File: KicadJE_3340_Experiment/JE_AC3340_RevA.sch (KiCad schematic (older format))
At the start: 89 parts

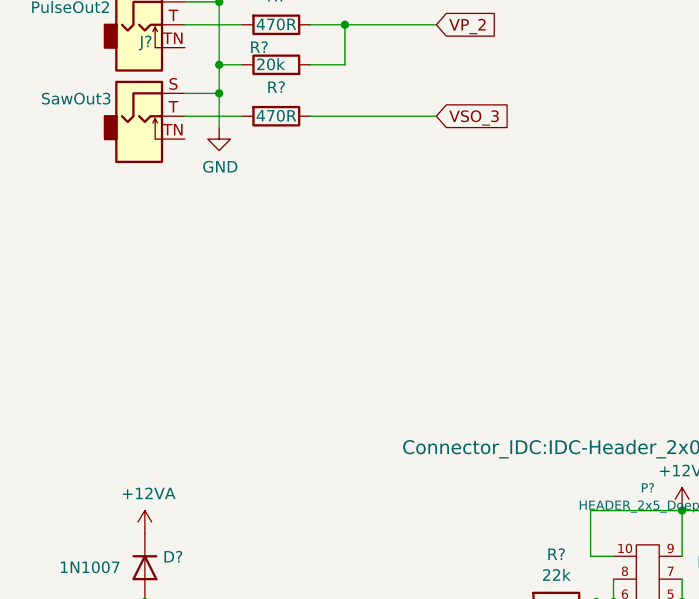
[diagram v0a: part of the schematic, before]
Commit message: Octave switch JE
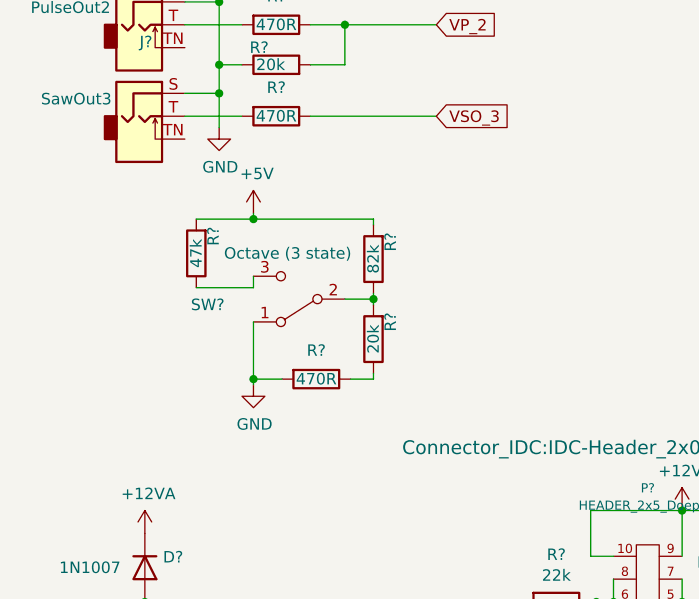
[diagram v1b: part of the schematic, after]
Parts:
- added R?: 82k, Resistor_SMD:R_0805_2012Metric_Pad1.15x1.40mm_HandSolder, symbol Device:R
- added R?: 20k, Resistor_SMD:R_0805_2012Metric_Pad1.15x1.40mm_HandSolder, symbol Device:R
- added R?: 47k, Resistor_SMD:R_0805_2012Metric_Pad1.15x1.40mm_HandSolder, symbol Device:R
- added R?: 470R, Resistor_SMD:R_0805_2012Metric_Pad1.15x1.40mm_HandSolder, symbol Device:R
- added SW?: Octave (3 state), AJ-Dropbox-Kicad:SP1MS1, symbol Switch:SW_SPDT
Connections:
- net +5V: now also R?.2, R?.2
- net GND: now also R?.2, SW?.1 (A)
- new net: R?.1, R?.2, SW?.2 (B)
- new net: R?.1, SW?.3 (C)
- new net: R?.1, R?.1
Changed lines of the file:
@@
 AR Path="/5E4B0DD9/5F66CD2B" Ref="U?"  Part="1"
 AR Path="/5E62ACA1/5F66CD2B" Ref="U?"  Part="1"
+AR Path="/5F49A670/5F66CD2B" Ref="U?"  Part="1"
 F 0 "U?" H 10300 4631 50  0000 C CNN
 F 1 "AS3340" H 10300 4540 50  0000 C CNN
@@
 AR Path="/5E4B0DD9/5F66CD3F" Ref="C?"  Part="1"
 AR Path="/5E62ACA1/5F66CD3F" Ref="C?"  Part="1"
+AR Path="/5F49A670/5F66CD3F" Ref="C?"  Part="1"
 F 0 "C?" H 9200 4450 50  0000 L CNN
 F 1 "1n poly" H 9125 4200 50  0000 L CNN
@@
 AR Path="/5E4B0DD9/5F66CD4A" Ref="R?"  Part="1"
 AR Path="/5E62ACA1/5F66CD4A" Ref="R?"  Part="1"
+AR Path="/5F49A670/5F66CD4A" Ref="R?"  Part="1"
 F 0 "R?" V 9550 4450 50  0000 C CNN
 F 1 "1k82" V 9675 4450 50  0000 C CNN
@@
 AR Path="/5E4B0DD9/5F66CD58" Ref="#PWR?"  Part="1"
 AR Path="/5E62ACA1/5F66CD58" Ref="#PWR?"  Part="1"
+AR Path="/5F49A670/5F66CD58" Ref="#PWR?"  Part="1"
 F 0 "#PWR?" H 9425 4400 50  0001 C CNN
 F 1 "GND" H 9430 4477 50  0000 C CNN
@@
 AR Path="/5E4B0DD9/5F66CD63" Ref="R?"  Part="1"
 AR Path="/5E62ACA1/5F66CD63" Ref="R?"  Part="1"
+AR Path="/5F49A670/5F66CD63" Ref="R?"  Part="1"
 F 0 "R?" V 9375 3400 50  0000 C CNN
 F 1 "6k04" V 9425 3250 50  0000 C CNN
@@
 AR Path="/5E4B0DD9/5F66CD69" Ref="R?"  Part="1"
 AR Path="/5E62ACA1/5F66CD69" Ref="R?"  Part="1"
+AR Path="/5F49A670/5F66CD69" Ref="R?"  Part="1"
 F 0 "R?" V 9325 3275 50  0000 C CNN
 F 1 "26k7" V 9425 3150 50  0000 C CNN
@@
 AR Path="/5E4B0DD9/5F66CD6F" Ref="RV?"  Part="1"
 AR Path="/5E62ACA1/5F66CD6F" Ref="RV?"  Part="1"
+AR Path="/5F49A670/5F66CD6F" Ref="RV?"  Part="1"
 F 0 "RV?" V 9150 3050 50  0000 C CNN
 F 1 "5k" V 9025 3175 50  0000 C CNN
@@
 AR Path="/5E4B0DD9/5F66CD7D" Ref="#PWR?"  Part="1"
 AR Path="/5E62ACA1/5F66CD7D" Ref="#PWR?"  Part="1"
+AR Path="/5F49A670/5F66CD7D" Ref="#PWR?"  Part="1"
 F 0 "#PWR?" H 10400 4350 50  0001 C CNN
 F 1 "GND" H 10405 4427 50  0000 C CNN
@@
 AR Path="/5E4B0DD9/5F66CD91" Ref="R?"  Part="1"
 AR Path="/5E62ACA1/5F66CD91" Ref="R?"  Part="1"
+AR Path="/5F49A670/5F66CD91" Ref="R?"  Part="1"
 F 0 "R?" V 9375 3500 50  0000 C CNN
 F 1 "1M2" V 9425 3350 50  0000 C CNN
@@
 U 1 1 5F66CD99
 P 8675 3150
+AR Path="/5E62ACA1/5F66CD99" Ref="#PWR?"  Part="1"
+AR Path="/5F49A670/5F66CD99" Ref="#PWR?"  Part="1"
 F 0 "#PWR?" H 8675 3250 50  0001 C CNN
 F 1 "-5V" H 8690 3323 50  0000 C CNN
@@
 AR Path="/5E4B0DD9/5F66CD9F" Ref="#PWR?"  Part="1"
 AR Path="/5E62ACA1/5F66CD9F" Ref="#PWR?"  Part="1"
+AR Path="/5F49A670/5F66CD9F" Ref="#PWR?"  Part="1"
 F 0 "#PWR?" H 9125 3225 50  0001 C CNN
 F 1 "-12VA" H 9140 3548 50  0000 C CNN
@@
 AR Path="/5F18E4B5/5F66CDA9" Ref="C?"  Part="1"
 AR Path="/5E62ACA1/5F66CDA9" Ref="C?"  Part="1"
+AR Path="/5F49A670/5F66CDA9" Ref="C?"  Part="1"
 F 0 "C?" H 8925 4450 50  0000 L CNN
 F 1 "100n" H 8850 4275 50  0000 L CNN
@@
 U 1 1 5F66CDB6
 P 10300 4625
+AR Path="/5E62ACA1/5F66CDB6" Ref="#PWR?"  Part="1"
+AR Path="/5F49A670/5F66CDB6" Ref="#PWR?"  Part="1"
 F 0 "#PWR?" H 10300 4725 50  0001 C CNN
 F 1 "-5V" H 10315 4798 50  0000 C CNN
@@
 U 1 1 5F66CDBC
 P 8550 3950
+AR Path="/5E62ACA1/5F66CDBC" Ref="Q?"  Part="1"
+AR Path="/5F49A670/5F66CDBC" Ref="Q?"  Part="1"
 F 0 "Q?" H 8741 3904 50  0000 L CNN
 F 1 "MMBT3906" H 8741 3995 50  0000 L CNN
@@
 AR Path="/5E4B0DD9/5F66CDC3" Ref="C?"  Part="1"
 AR Path="/5E62ACA1/5F66CDC3" Ref="C?"  Part="1"
+AR Path="/5F49A670/5F66CDC3" Ref="C?"  Part="1"
 F 0 "C?" V 7550 4150 50  0000 L CNN
 F 1 "220p" V 7650 4150 50  0000 L CNN
@@
 AR Path="/5E4B0DD9/5F66CDC9" Ref="R?"  Part="1"
 AR Path="/5E62ACA1/5F66CDC9" Ref="R?"  Part="1"
+AR Path="/5F49A670/5F66CDC9" Ref="R?"  Part="1"
 F 0 "R?" V 7900 4025 50  0000 C CNN
 F 1 "47k" V 8000 4100 50  0000 C CNN
@@
 AR Path="/5E4B0DD9/5F66CDD1" Ref="R?"  Part="1"
 AR Path="/5E62ACA1/5F66CDD1" Ref="R?"  Part="1"
+AR Path="/5F49A670/5F66CDD1" Ref="R?"  Part="1"
 F 0 "R?" V 8125 3725 50  0000 C CNN
 F 1 "47k" V 8225 3800 50  0000 C CNN
@@
 U 1 1 5F66CDDA
 P 7975 3400
+AR Path="/5E62ACA1/5F66CDDA" Ref="#PWR?"  Part="1"
+AR Path="/5F49A670/5F66CDDA" Ref="#PWR?"  Part="1"
 F 0 "#PWR?" H 7975 3250 50  0001 C CNN
 F 1 "+5V" H 7990 3573 50  0000 C CNN
@@
 AR Path="/5F18E4B5/5F66CDE3" Ref="C?"  Part="1"
 AR Path="/5E62ACA1/5F66CDE3" Ref="C?"  Part="1"
+AR Path="/5F49A670/5F66CDE3" Ref="C?"  Part="1"
 F 0 "C?" H 8650 4450 50  0000 L CNN
 F 1 "100n" H 8550 4275 50  0000 L CNN
@@
 U 1 1 5F66CDEE
 P 8425 4175
+AR Path="/5E62ACA1/5F66CDEE" Ref="D?"  Part="1"
+AR Path="/5F49A670/5F66CDEE" Ref="D?"  Part="1"
 F 0 "D?" H 8325 4250 50  0000 C CNN
 F 1 "Germanium" H 8325 4100 50  0000 C CNN
@@
 U 1 1 5F66CDFA
 P 8225 3450
+AR Path="/5E62ACA1/5F66CDFA" Ref="JP?"  Part="1"
+AR Path="/5F49A670/5F66CDFA" Ref="JP?"  Part="1"
 F 0 "JP?" H 8225 3654 50  0000 C CNN
 F 1 "Jumper_3_Bridged12" H 8225 3563 50  0000 C CNN
@@
 	1    0    0    -1
 $EndComp
+$Comp
+L Switch:SW_SPDT SW?
+U 1 1 5F6B865F
+P 1700 5675
+AR Path="/5F6B865F" Ref="SW?"  Part="1"
+AR Path="/5C8C5FC0/5F6B865F" Ref="SW?"  Part="1"
+AR Path="/5CAAE8D3/5F6B865F" Ref="SW?"  Part="1"
+AR Path="/5E4B0DD9/5F6B865F" Ref="SW?"  Part="1"
+AR Path="/5E62ACA1/5F6B865F" Ref="SW?"  Part="1"
+AR Path="/5F49A670/5F6B865F" Ref="SW?"  Part="1"
+F 0 "SW?" H 2100 5700 50  0000 C CNN
+F 1 "Octave (3 state)" H 1750 5475 50  0000 C CNN
+F 2 "AJ-Dropbox-Kicad:SP1MS1" H 1700 5675 50  0001 C CNN
+F 3 "~" H 1700 5675 50  0001 C CNN
+	1    1700 5675
+	-1   0    0    1
+$EndComp
+$Comp
+L Envelope-cache-2018-08-04-13-00-04:+5V #PWR?
+U 1 1 5F6F74CC
+P 1500 5300
+AR Path="/5E62ACA1/5F6F74CC" Ref="#PWR?"  Part="1"
+AR Path="/5F49A670/5F6F74CC" Ref="#PWR?"  Part="1"
+F 0 "#PWR?" H 1500 5150 50  0001 C CNN
+F 1 "+5V" H 1515 5473 50  0000 C CNN
+F 2 "" H 1500 5300 50  0001 C CNN
+F 3 "" H 1500 5300 50  0001 C CNN
+	1    1500 5300
+	1    0    0    -1
+$EndComp
+$Comp
+L Device:R R?
+U 1 1 5F6F7A40
+P 2025 5500
+AR Path="/5F6F7A40" Ref="R?"  Part="1"
+AR Path="/5C8C5FC0/5F6F7A40" Ref="R?"  Part="1"
+AR Path="/5CAAE8D3/5F6F7A40" Ref="R?"  Part="1"
+AR Path="/5E4B0DD9/5F6F7A40" Ref="R?"  Part="1"
+AR Path="/5E62ACA1/5F6F7A40" Ref="R?"  Part="1"
+AR Path="/5F49A670/5F6F7A40" Ref="R?"  Part="1"
+F 0 "R?" V 1950 5425 50  0000 C CNN
+F 1 "82k" V 2025 5500 50  0000 C CNN
+F 2 "Resistor_SMD:R_0805_2012Metric_Pad1.15x1.40mm_HandSolder" V 1955 5500 50  0001 C CNN
+F 3 "~" H 2025 5500 50  0001 C CNN
+	1    2025 5500
+	-1   0    0    1
+$EndComp
+$Comp
+L Device:R R?
+U 1 1 5F6F8705
+P 2025 5850
+AR Path="/5F6F8705" Ref="R?"  Part="1"
+AR Path="/5C8C5FC0/5F6F8705" Ref="R?"  Part="1"
+AR Path="/5CAAE8D3/5F6F8705" Ref="R?"  Part="1"
+AR Path="/5E4B0DD9/5F6F8705" Ref="R?"  Part="1"
+AR Path="/5E62ACA1/5F6F8705" Ref="R?"  Part="1"
+AR Path="/5F49A670/5F6F8705" Ref="R?"  Part="1"
+F 0 "R?" V 1950 5775 50  0000 C CNN
+F 1 "20k" V 2025 5850 50  0000 C CNN
+F 2 "Resistor_SMD:R_0805_2012Metric_Pad1.15x1.40mm_HandSolder" V 1955 5850 50  0001 C CNN
+F 3 "~" H 2025 5850 50  0001 C CNN
+	1    2025 5850
+	-1   0    0    1
+$EndComp
+$Comp
+L Envelope-cache-2018-08-04-13-00-04:GND #PWR?
+U 1 1 5F6F8CBF
+P 1500 6050
+AR Path="/5F6F8CBF" Ref="#PWR?"  Part="1"
+AR Path="/5C8C5FC0/5F6F8CBF" Ref="#PWR?"  Part="1"
+AR Path="/5CAAE8D3/5F6F8CBF" Ref="#PWR?"  Part="1"
+AR Path="/5E4B0DD9/5F6F8CBF" Ref="#PWR?"  Part="1"
+AR Path="/5F49A670/5F6F8CBF" Ref="#PWR?"  Part="1"
+F 0 "#PWR?" H 1500 5800 50  0001 C CNN
+F 1 "GND" H 1505 5877 50  0000 C CNN
+F 2 "" H 1500 6050 50  0001 C CNN
+F 3 "" H 1500 6050 50  0001 C CNN
+	1    1500 6050
+	1    0    0    -1
+$EndComp
+Wire Wire Line
+	2025 5350 2025 5325
+Wire Wire Line
+	2025 5325 1500 5325
+Wire Wire Line
+	1500 5325 1500 5300
+Wire Wire Line
+	1500 6050 1500 6025
+Wire Wire Line
+	1500 6025 1625 6025
+Wire Wire Line
+	2025 6025 2025 6000
+Wire Wire Line
+	2025 5700 2025 5675
+Wire Wire Line
+	1900 5675 2025 5675
+Connection ~ 2025 5675
+Wire Wire Line
+	2025 5675 2025 5650
+$Comp
+L Device:R R?
+U 1 1 5F753A2A
+P 1250 5475
+AR Path="/5F753A2A" Ref="R?"  Part="1"
+AR Path="/5C8C5FC0/5F753A2A" Ref="R?"  Part="1"
+AR Path="/5CAAE8D3/5F753A2A" Ref="R?"  Part="1"
+AR Path="/5E4B0DD9/5F753A2A" Ref="R?"  Part="1"
+AR Path="/5E62ACA1/5F753A2A" Ref="R?"  Part="1"
+AR Path="/5F49A670/5F753A2A" Ref="R?"  Part="1"
+F 0 "R?" V 1175 5400 50  0000 C CNN
+F 1 "47k" V 1250 5475 50  0000 C CNN
+F 2 "Resistor_SMD:R_0805_2012Metric_Pad1.15x1.40mm_HandSolder" V 1180 5475 50  0001 C CNN
+F 3 "~" H 1250 5475 50  0001 C CNN
+	1    1250 5475
+	-1   0    0    1
+$EndComp
+Wire Wire Line
+	1250 5325 1500 5325
+Connection ~ 1500 5325
+Wire Wire Line
+	1250 5625 1500 5625
+Wire Wire Line
+	1500 5625 1500 5575
+Wire Wire Line
+	1500 5775 1500 6025
+Connection ~ 1500 6025
+$Comp
+L Device:R R?
+U 1 1 5F79A77D
+P 1775 6025
+AR Path="/5F79A77D" Ref="R?"  Part="1"
+AR Path="/5C8C5FC0/5F79A77D" Ref="R?"  Part="1"
+AR Path="/5CAAE8D3/5F79A77D" Ref="R?"  Part="1"
+AR Path="/5E4B0DD9/5F79A77D" Ref="R?"  Part="1"
+AR Path="/5F49A670/5F79A77D" Ref="R?"  Part="1"
+F 0 "R?" V 1650 6025 50  0000 C CNN
+F 1 "470R" V 1775 6025 50  0000 C CNN
+F 2 "Resistor_SMD:R_0805_2012Metric_Pad1.15x1.40mm_HandSolder" V 1705 6025 50  0001 C CNN
+F 3 "~" H 1775 6025 50  0001 C CNN
+	1    1775 6025
+	0    1    1    0
+$EndComp
+Wire Wire Line
+	1925 6025 2025 6025
 $EndSCHEMATC
